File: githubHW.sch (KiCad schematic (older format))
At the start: 142 parts, among them J1 Conn_01x06, J2 Conn_01x07, J3 Conn_01x07, J4 Conn_01x07, J5 Conn_01x07, J6 Conn_01x06, SW1 SW_Push, SW2 SW_Push, SW3 SW_Push, SW4 SW_Push, U1 WeMos_mini, U2 TPIC6B595N, U3 TLC5940NT, U4 TPIC6B595N

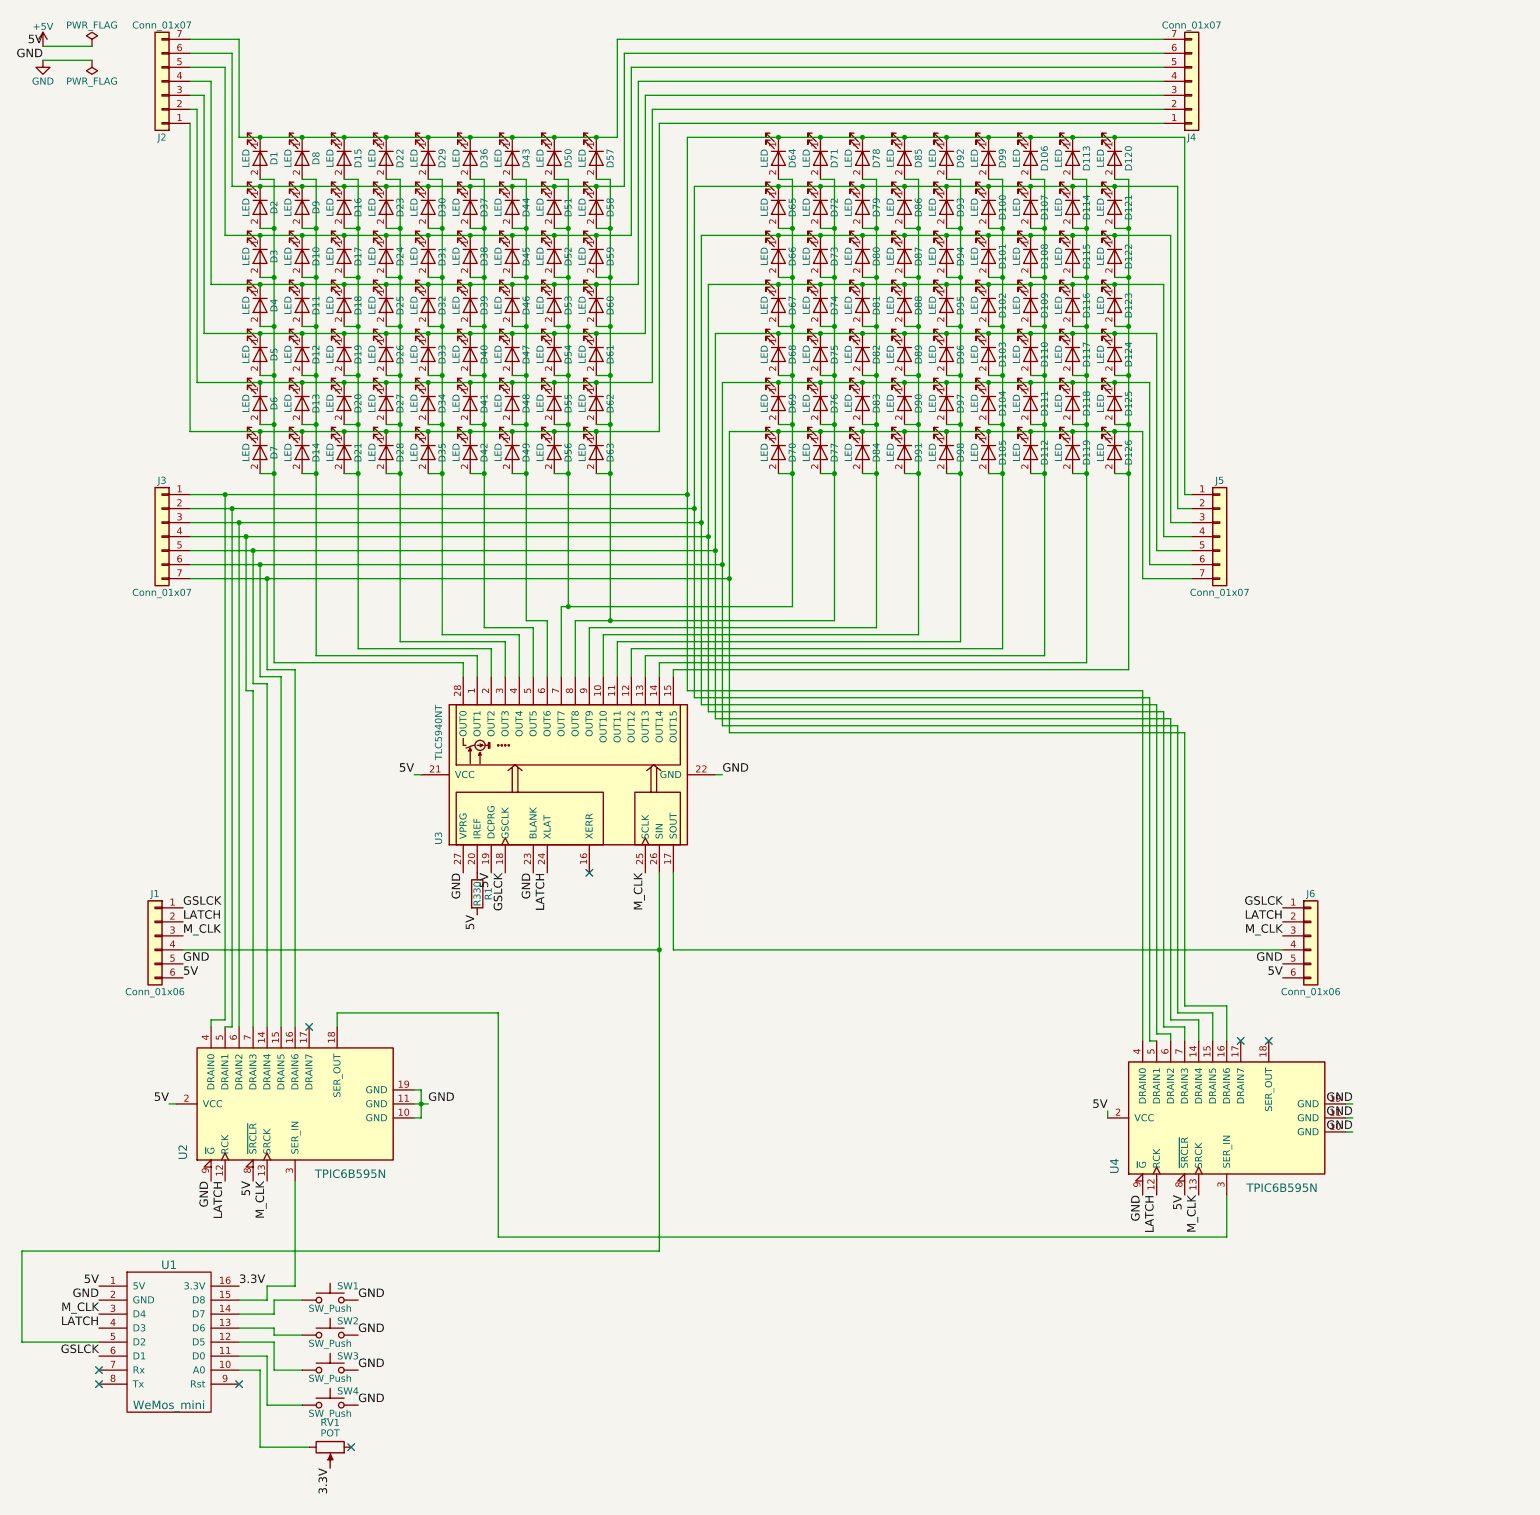
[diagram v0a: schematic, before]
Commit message: Revert "connection issue fixed"
This reverts commit d7eb6beb1c8d570a5e8c06e88c024579e6cb722b.
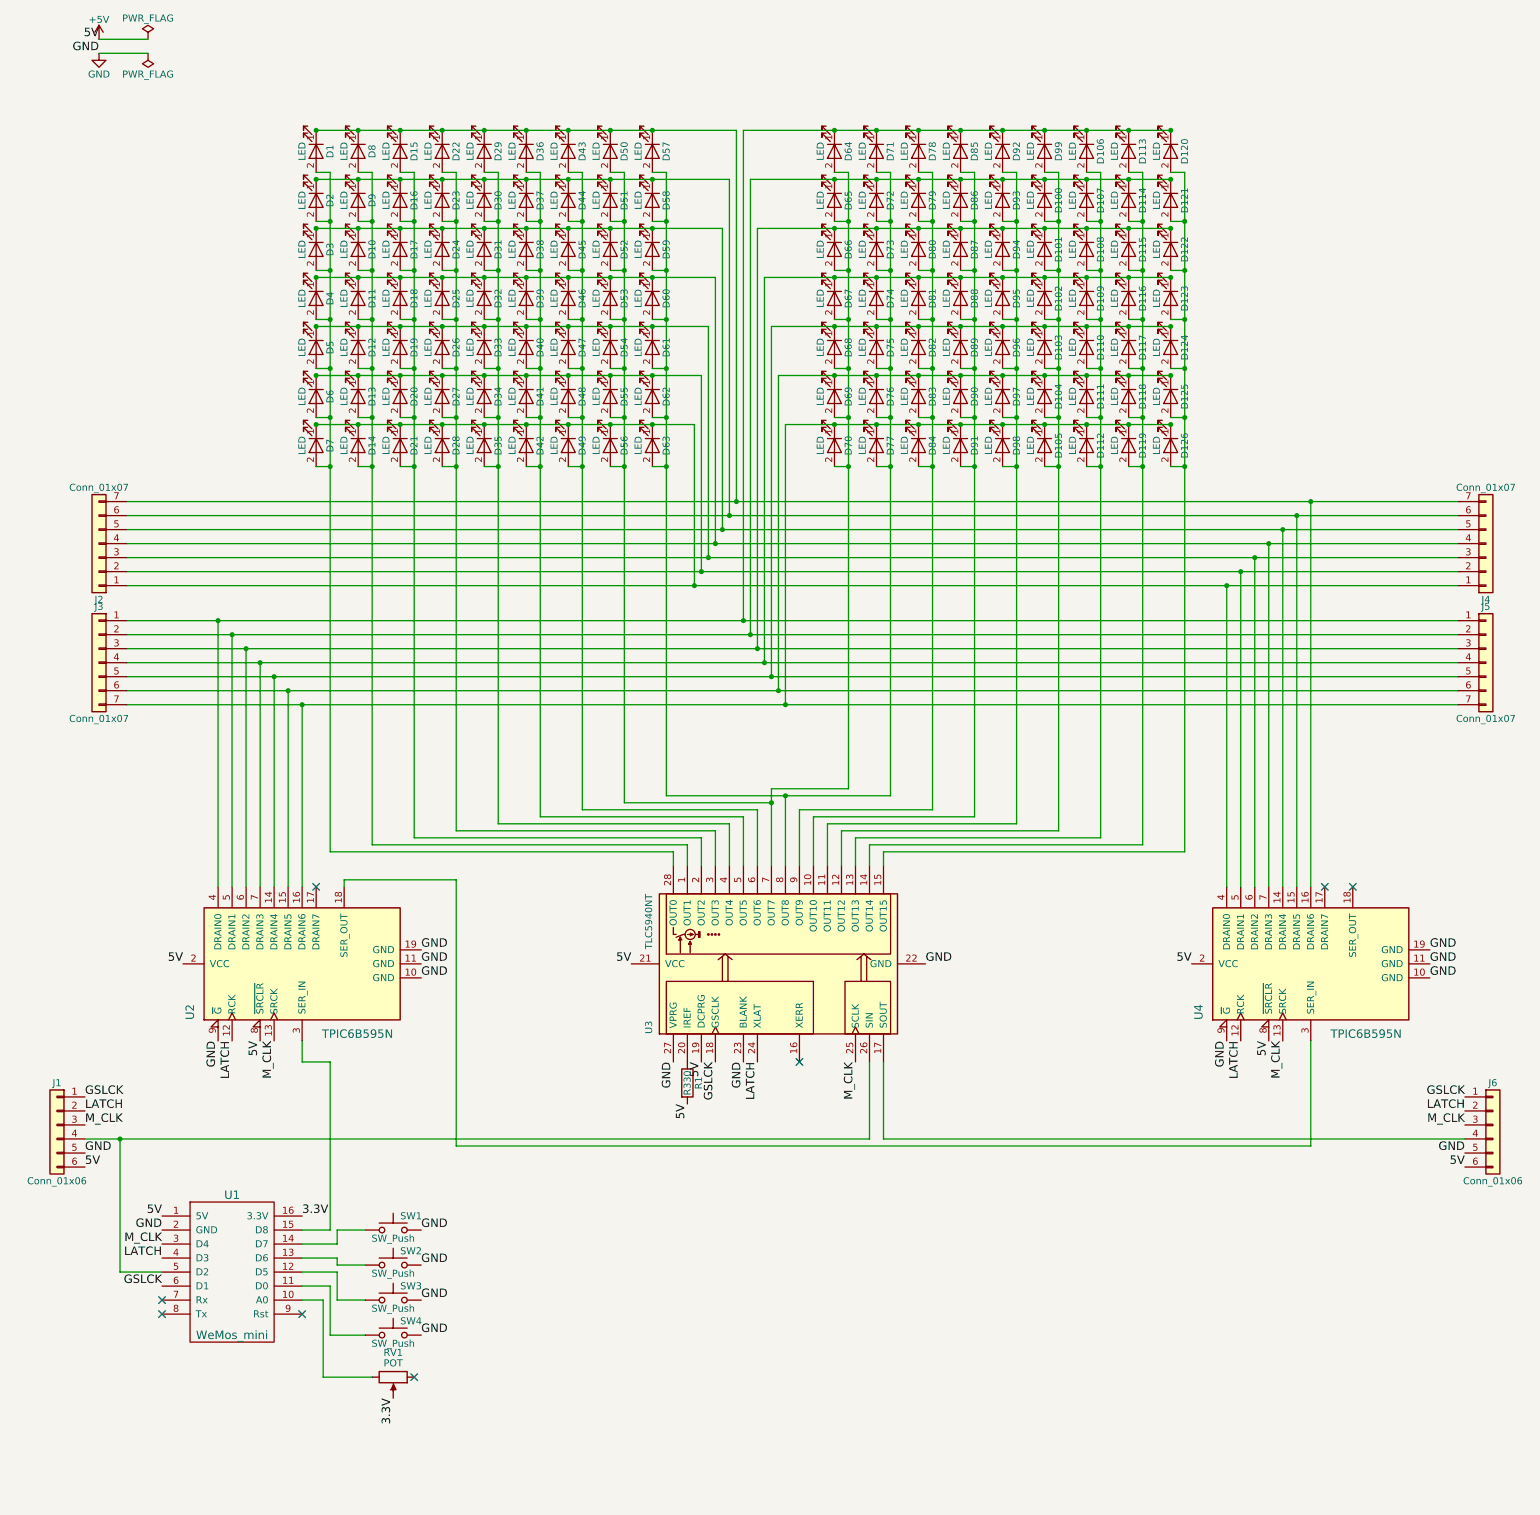
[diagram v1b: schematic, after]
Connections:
- net at D100.1 (K), D107.1 (K), D114.1 (K)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: no longer U4.5 (DRAIN1)
- net at D106.1 (K), D113.1 (K), D120.1 (K)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: no longer U4.4 (DRAIN0)
- net at D101.1 (K), D108.1 (K), D115.1 (K)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: no longer U4.6 (DRAIN2)
- net at D102.1 (K), D109.1 (K), D116.1 (K)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: no longer U4.7 (DRAIN3)
- net at D103.1 (K), D110.1 (K), D117.1 (K)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: no longer U4.14 (DRAIN4)
- net at D104.1 (K), D111.1 (K), D118.1 (K)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: no longer U4.15 (DRAIN5)
- net at D105.1 (K), D112.1 (K), D119.1 (K)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: no longer U4.16 (DRAIN6)
- net at D16.1 (K), D2.1 (K), D23.1 (K)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: now also U4.15 (DRAIN5)
- net at D1.1 (K), D15.1 (K), D22.1 (K)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: now also U4.16 (DRAIN6)
- net at D10.1 (K), D17.1 (K), D24.1 (K)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: now also U4.14 (DRAIN4)
- net at D11.1 (K), D18.1 (K), D25.1 (K)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: now also U4.7 (DRAIN3)
- net at D12.1 (K), D19.1 (K), D26.1 (K)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: now also U4.6 (DRAIN2)
- net at D13.1 (K), D20.1 (K), D27.1 (K)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: now also U4.5 (DRAIN1)
- net at D14.1 (K), D21.1 (K), D28.1 (K)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: now also U4.4 (DRAIN0)
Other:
- moved on the sheet: D1, D10, D100, D101, D102, D103, D104, D105, D106, D107, D108, D109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
